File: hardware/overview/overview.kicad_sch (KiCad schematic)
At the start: 0 parts

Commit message: hmm. kicad and git dont play well together
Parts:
- added U1: (no value), symbol kl_parts:kl_amistar_hio1
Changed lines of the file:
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@@
 	(generator_version "10.0")
 	(paper "A4")
+	(symbol
+		(lib_id "kl_parts:kl_amistar_hio1")
+		(at 90.17 129.54 0)
+		(unit 1)
+		(body_style 1)
+		(exclude_from_sim no)
+		(in_bom yes)
+		(on_board yes)
+		(in_pos_files yes)
+		(dnp no)
+		(fields_autoplaced yes)
+		(property "Reference" "U1"
+			(at 96.52 105.4099 0)
+			(show_name no)
+			(do_not_autoplace no)
+			(effects
+				(font
+					(size 1.27 1.27)
+				)
+				(justify left)
+			)
+		)
+		(property "Value" ""
+			(at 90.17 129.54 0)
+			(show_name no)
+			(do_not_autoplace no)
+			(effects
+				(font
+					(size 1.27 1.27)
+				)
+			)
+		)
+		(property "Footprint" ""
+			(at 90.17 129.54 0)
+			(hide yes)
+			(show_name no)
+			(do_not_autoplace no)
+			(effects
+				(font
+					(size 1.27 1.27)
+				)
+			)
+		)
+		(property "Datasheet" ""
+			(at 90.17 129.54 0)
+			(hide yes)
+			(show_name no)
+			(do_not_autoplace no)
+			(effects
+				(font
+					(size 1.27 1.27)
+				)
+			)
+		)
+		(property "Description" ""
+			(at 90.17 129.54 0)
+			(hide yes)
+			(show_name no)
+			(do_not_autoplace no)
+			(effects
+				(font
+					(size 1.27 1.27)
+				)
+			)
+		)
+		(pin ""
+		)
+		(instances
+			(project "overview"
+				(path "/d999ca8c-b4a1-4c29-819a-63809fda4f99"
+					(reference "U1")
+					(unit 1)
+				)
+			)
+		)
+	)
 	(sheet_instances
 		(path "/"

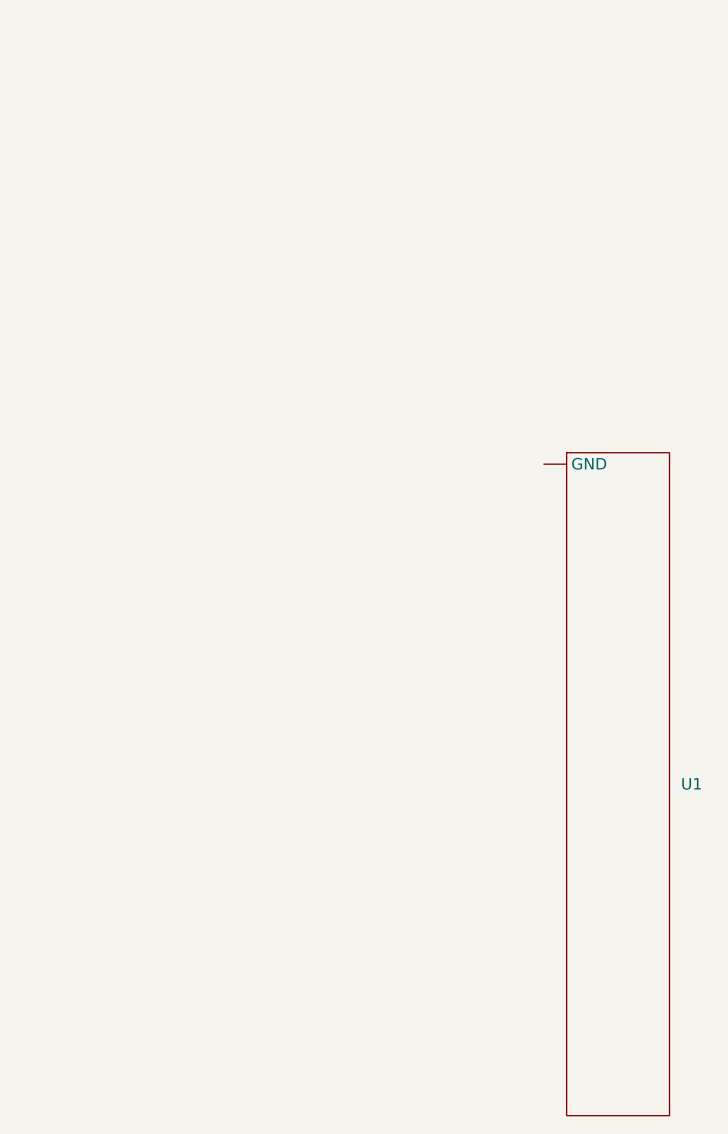
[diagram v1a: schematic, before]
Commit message: remembering how to use kicad
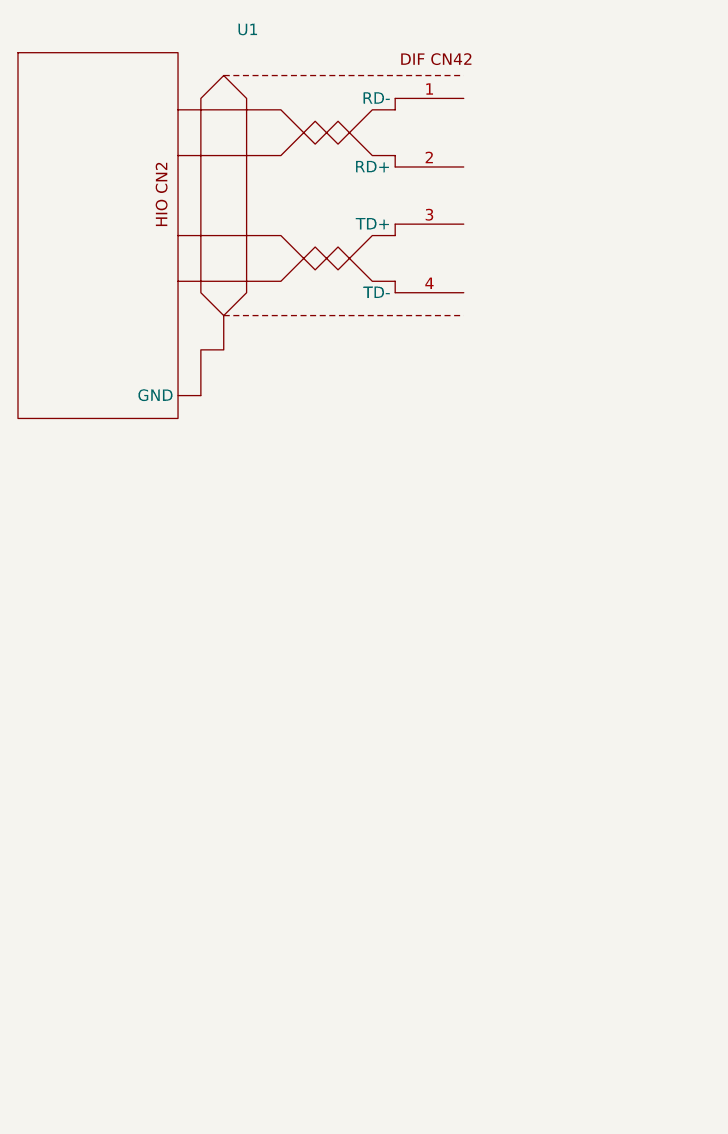
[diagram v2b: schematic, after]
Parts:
- removed U1: (no value), symbol kl_parts:kl_amistar_hio1
- added U1: (no value), symbol kl_parts:kl_amistar_hio_CN2
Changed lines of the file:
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@@
 	(paper "A4")
 	(symbol
-		(lib_id "kl_parts:kl_amistar_hio1")
-		(at 90.17 129.54 0)
+		(lib_id "kl_parts:kl_amistar_hio_CN2")
+		(at 44.45 87.63 0)
 		(unit 1)
 		(body_style 1)
@@
 		(fields_autoplaced yes)
 		(property "Reference" "U1"
-			(at 96.52 105.4099 0)
+			(at 48.3942 21.59 0)
 			(show_name no)
 			(do_not_autoplace no)
@@
 					(size 1.27 1.27)
 				)
-				(justify left)
 			)
 		)
 		(property "Value" ""
-			(at 90.17 129.54 0)
+			(at 44.45 87.63 0)
 			(show_name no)
 			(do_not_autoplace no)
@@
 		)
 		(property "Footprint" ""
-			(at 90.17 129.54 0)
+			(at 44.45 87.63 0)
 			(hide yes)
 			(show_name no)
@@
 		)
 		(property "Datasheet" ""
-			(at 90.17 129.54 0)
+			(at 44.45 87.63 0)
 			(hide yes)
 			(show_name no)
@@
 		)
 		(property "Description" ""
-			(at 90.17 129.54 0)
+			(at 44.45 87.63 0)
 			(hide yes)
 			(show_name no)
@@
 			)
 		)
+		(pin "4"
+		)
+		(pin "1"
+		)
 		(pin ""
 		)
+		(pin "2"
+		)
+		(pin "3"
+		)
 		(instances

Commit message: schematics
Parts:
- removed U1: (no value), symbol kl_parts:kl_amistar_hio_CN2
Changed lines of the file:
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@@
 	(generator_version "10.0")
 	(paper "A4")
-	(symbol
-		(lib_id "kl_parts:kl_amistar_hio_CN2")
-		(at 44.45 87.63 0)
-		(unit 1)
-		(body_style 1)
-		(exclude_from_sim no)
-		(in_bom yes)
-		(on_board yes)
-		(in_pos_files yes)
-		(dnp no)
-		(fields_autoplaced yes)
-		(property "Reference" "U1"
-			(at 48.3942 21.59 0)
-			(show_name no)
-			(do_not_autoplace no)
-			(effects
-				(font
-					(size 1.27 1.27)
-				)
-			)
-		)
-		(property "Value" ""
-			(at 44.45 87.63 0)
-			(show_name no)
-			(do_not_autoplace no)
-			(effects
-				(font
-					(size 1.27 1.27)
-				)
-			)
-		)
-		(property "Footprint" ""
-			(at 44.45 87.63 0)
-			(hide yes)
-			(show_name no)
-			(do_not_autoplace no)
-			(effects
-				(font
-					(size 1.27 1.27)
-				)
-			)
-		)
-		(property "Datasheet" ""
-			(at 44.45 87.63 0)
-			(hide yes)
-			(show_name no)
-			(do_not_autoplace no)
-			(effects
-				(font
-					(size 1.27 1.27)
-				)
-			)
-		)
-		(property "Description" ""
-			(at 44.45 87.63 0)
-			(hide yes)
-			(show_name no)
-			(do_not_autoplace no)
-			(effects
-				(font
-					(size 1.27 1.27)
-				)
-			)
-		)
-		(pin "4"
-		)
-		(pin "1"
-		)
-		(pin ""
-		)
-		(pin "2"
-		)
-		(pin "3"
-		)
-		(instances
-			(project "overview"
-				(path "/d999ca8c-b4a1-4c29-819a-63809fda4f99"
-					(reference "U1")
-					(unit 1)
-				)
-			)
-		)
-	)
 	(sheet_instances
 		(path "/"
